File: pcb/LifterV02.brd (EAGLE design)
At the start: 109.2 x 25 mm, 60 parts, among them IC2 TL072D

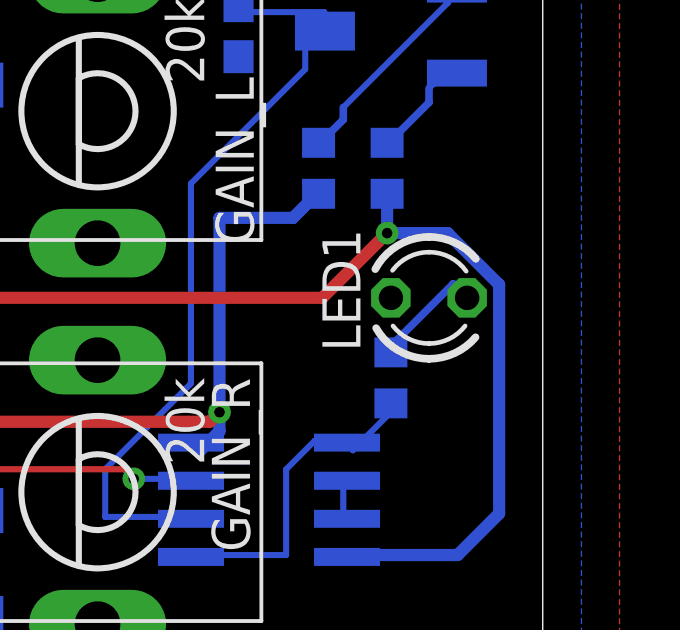
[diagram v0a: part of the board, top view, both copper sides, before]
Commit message: BigMac changes.
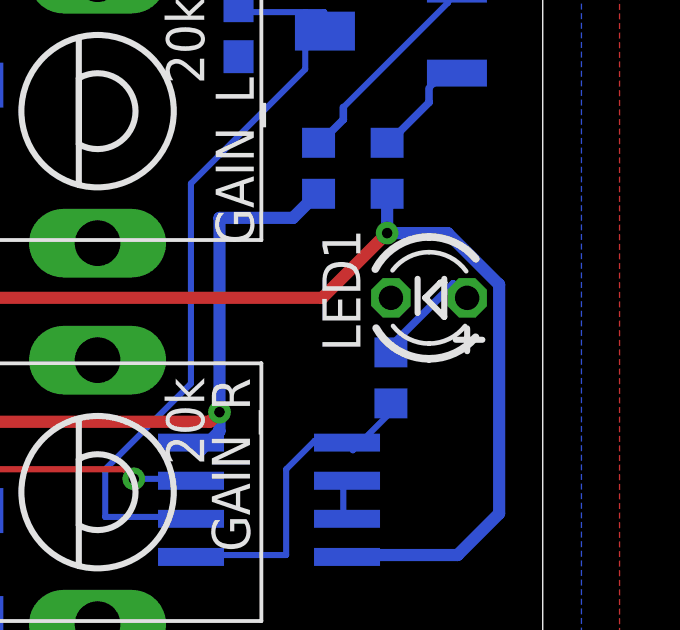
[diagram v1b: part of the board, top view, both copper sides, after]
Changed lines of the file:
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@@
 <layer number="23" name="tOrigins" color="15" fill="1" visible="no" active="yes"/>
 <layer number="24" name="bOrigins" color="15" fill="1" visible="yes" active="yes"/>
-<layer number="25" name="tNames" color="7" fill="1" visible="no" active="yes"/>
+<layer number="25" name="tNames" color="7" fill="1" visible="yes" active="yes"/>
 <layer number="26" name="bNames" color="7" fill="1" visible="yes" active="yes"/>
 <layer number="27" name="tValues" color="7" fill="1" visible="no" active="yes"/>
@@
 <circle x="57.912" y="16.383" radius="0.283978125" width="0.4064" layer="26"/>
 <circle x="99.314" y="4.191" radius="0.283978125" width="0.4064" layer="26"/>
+<wire x1="105.918" y1="13.335" x2="105.918" y2="13.208" width="0.2032" layer="25"/>
+<wire x1="105.918" y1="13.208" x2="105.918" y2="12.065" width="0.2032" layer="25"/>
+<wire x1="105.918" y1="12.065" x2="105.283" y2="12.7" width="0.2032" layer="25"/>
+<wire x1="105.283" y1="12.7" x2="105.791" y2="13.208" width="0.2032" layer="25"/>
+<wire x1="105.791" y1="13.208" x2="105.918" y2="13.208" width="0.2032" layer="25"/>
+<wire x1="105.029" y1="13.335" x2="105.029" y2="12.192" width="0.2032" layer="25"/>
+<wire x1="107.188" y1="11.303" x2="106.299" y2="11.303" width="0.2032" layer="25"/>
+<wire x1="106.68" y1="11.684" x2="106.68" y2="10.922" width="0.2032" layer="25"/>
 </plain>
 <attributes>
